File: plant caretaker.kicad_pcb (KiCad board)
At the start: 2 copper layers, 62.5 x 120.2 mm, 58 parts, among them J3 Water_Pump, J4 Kitronik, J5 694106402002, Q1 FDMS86255, U1 UDA1380HN_N2, U2 TMP175AIDR, U4 LM2596S-5, U5 PAM8403D, U6 ESP32_C3_ZERO

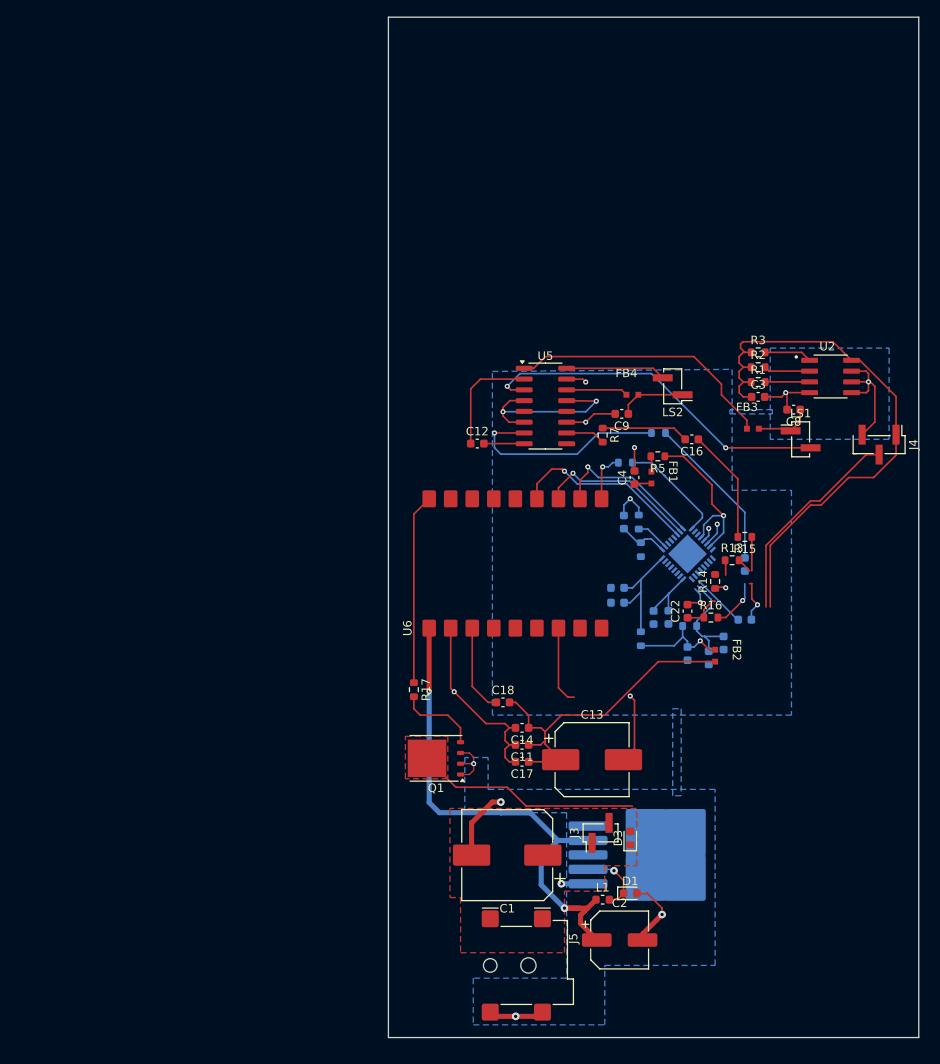
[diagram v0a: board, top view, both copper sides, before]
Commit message: Different version of connections
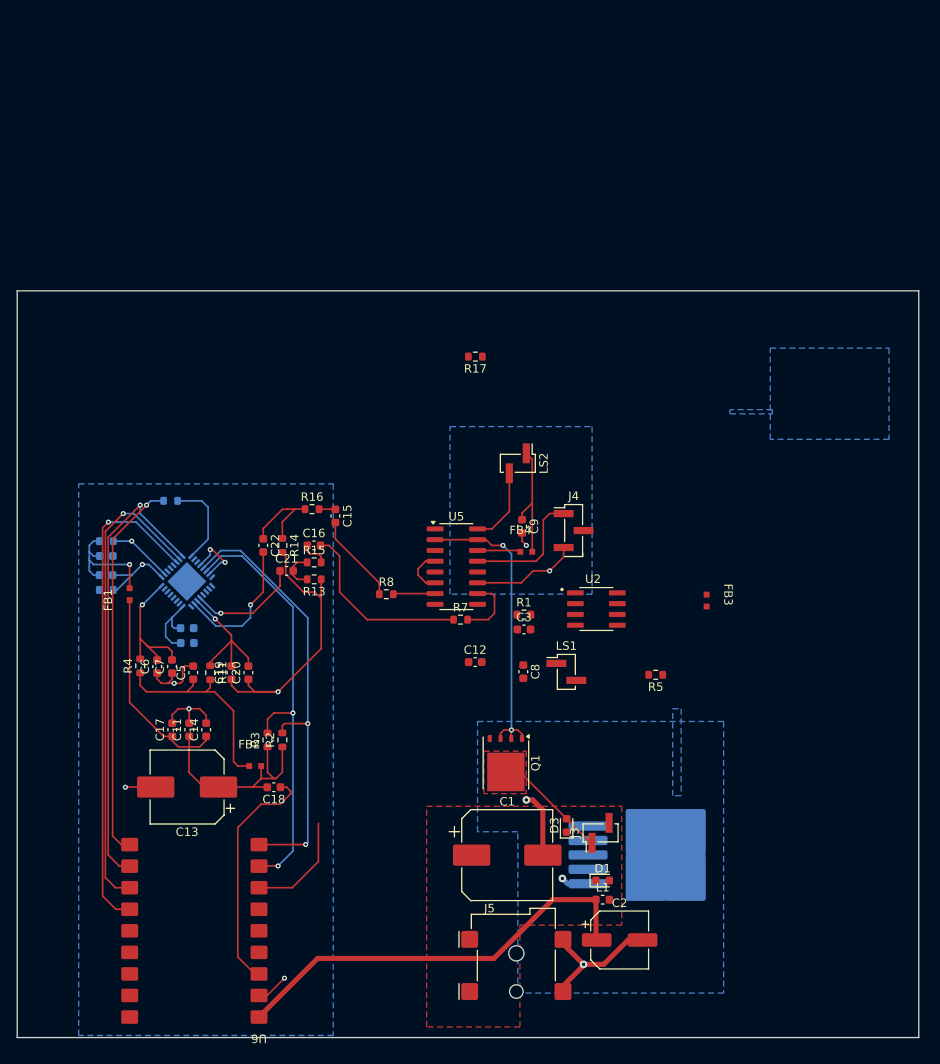
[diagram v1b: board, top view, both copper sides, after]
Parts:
- C15, C19, C20, C21, C5, C6, C7, R11, R4, R8: moved to F.Cu
- C4: moved to B.Cu
- moved R3 73.7 mm to (62.2, 110.2), turned to 90 degrees
- moved R2 71.2 mm to (64.0, 110.2), turned to 90 degrees
- moved FB1 63.3 mm to (46.0, 93.7), turned to 90 degrees
- moved R6 63.2 mm to (43.2, 92.5), turned to 0 degrees
- moved C4 62.9 mm to (43.2, 88.5), turned to 0 degrees
- moved R9 62.8 mm to (43.2, 86.8), turned to 180 degrees
- moved C10 61.3 mm to (43.2, 90.8), turned to 0 degrees
- moved U1 59.1 mm to (52.8, 91.5)
- moved R4 59.1 mm to (47.2, 101.5)
- moved C5 58.3 mm to (53.5, 102.2), turned to 90 degrees
- moved C19 58.1 mm to (58.0, 102.2)
- moved R11 56.8 mm to (55.5, 102.2), turned to -90 degrees
- moved C23 56.7 mm to (52.8, 97.0), turned to 180 degrees
- moved FB2 56.6 mm to (60.1, 113.2), turned to 0 degrees
- moved C24 55.0 mm to (52.8, 98.8), turned to 180 degrees
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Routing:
- net +3V3: track 129.5 -> 71.6 mm, vias 2 -> 0
- net /AudioCodec/SCL: track 7.10 -> 52.7 mm, vias 1 -> 2
- net /AudioCodec/SDA: track 8.43 -> 51.9 mm, vias 1 -> 2
- net Net-(U5-LOUT-): track 42.2 -> 0.00 mm, vias 2 -> 0
- net /CODEC.SYSCLK: track 5.87 -> 45.3 mm
- net /CODEC.WSI: track 19.2 -> 56.0 mm
- net /CODEC.BCKI: track 22.2 -> 58.2 mm
- net /CODEC.DATAI: track 18.4 -> 54.0 mm
- net Net-(U5-LOUT+): track 31.7 -> 0.00 mm
- net /BuckConverter/PWM_IN: track 22.4 -> 0.00 mm
- net GND: track 110.3 -> 132.2 mm
- net Net-(J4-Pin_2): track 34.4 -> 12.8 mm
- net Net-(U5-INL): track 25.1 -> 4.96 mm, vias 1 -> 0
- net Net-(U6-3V3_OUT): track 10.5 -> 28.2 mm
- net /AudioCodec/VDDA: track 12.1 -> 25.2 mm, vias 1 -> 0
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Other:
- board size 62.5 x 120.2 mm -> 106.2 x 88 mm
